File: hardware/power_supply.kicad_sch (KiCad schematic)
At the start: 38 parts, among them U201 PLMR51635XDDCR, U202 AP63203WU, U203 TPS62A04ADRL, U204 LP5910-1.8DRV

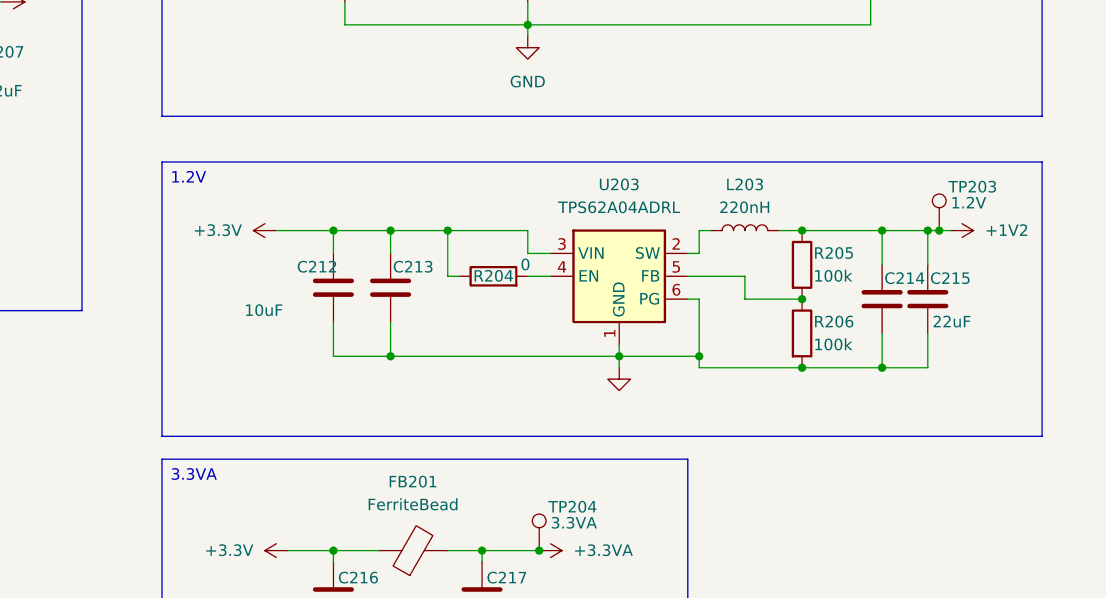
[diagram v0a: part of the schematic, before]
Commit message: ✨ Final PCB v.1 updates
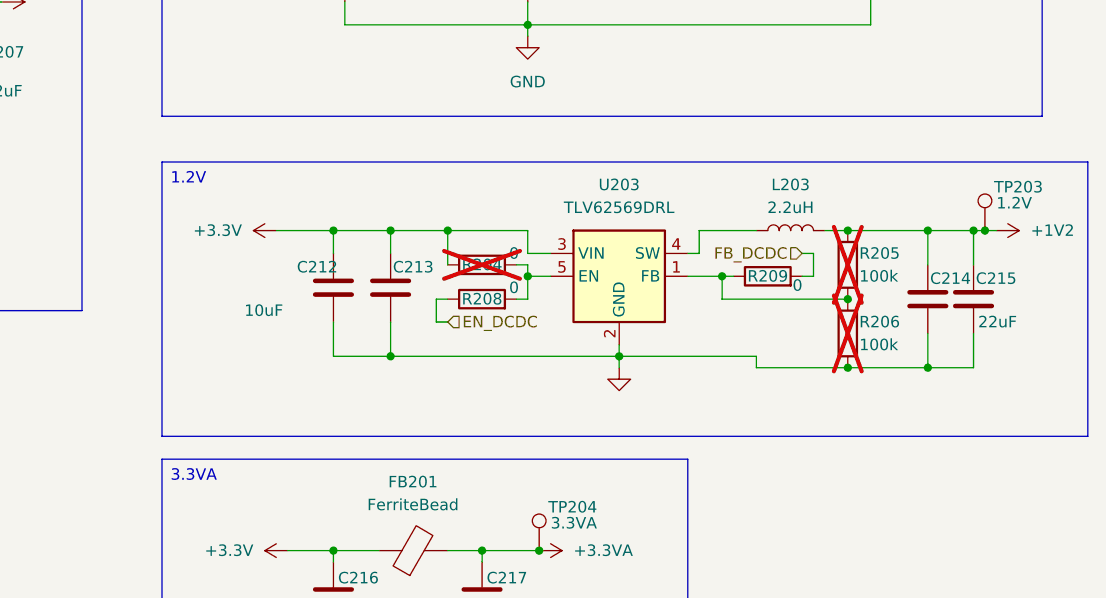
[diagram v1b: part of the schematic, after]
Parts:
- removed U203: TPS62A04ADRL, Package_TO_SOT_SMD:SOT-563, symbol Regulator_Switching:TPS62A01ADRL
- added R208, R209: 0, PCM_Resistor_SMD_AKL:R_0402_1005Metric, symbol Device:R
- added U203: TLV62569DRL, Package_TO_SOT_SMD:SOT-563, symbol Regulator_Switching:TLV62569DRL
- L203: value 220nH -> 2.2uH; footprint Inductor_SMD:L_0603_1608Metric -> PCM_Inductor_SMD_AKL:L_1008_2520Metric
- R204: now not fitted
- R205, R206: footprint Resistor_SMD:R_0603_1608Metric -> PCM_Resistor_SMD_AKL:R_0402_1005Metric; now not fitted
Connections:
- net +3.3V: now also U203.3 (VIN)
- net GND: now also U203.2 (GND)
- net at R204.2: now also R208.2, U203.5 (EN)
- net at L203.1: now also U203.4 (SW)
- net at R205.2, R206.1: now also R209.1, U203.1 (FB)
- new net EN_DCDC: R208.1
- new net FB_DCDC: R209.2
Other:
- moved on the sheet: C214, C215, L203, TP203
